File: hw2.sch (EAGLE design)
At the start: 23 parts, among them J1 USB-MB-H

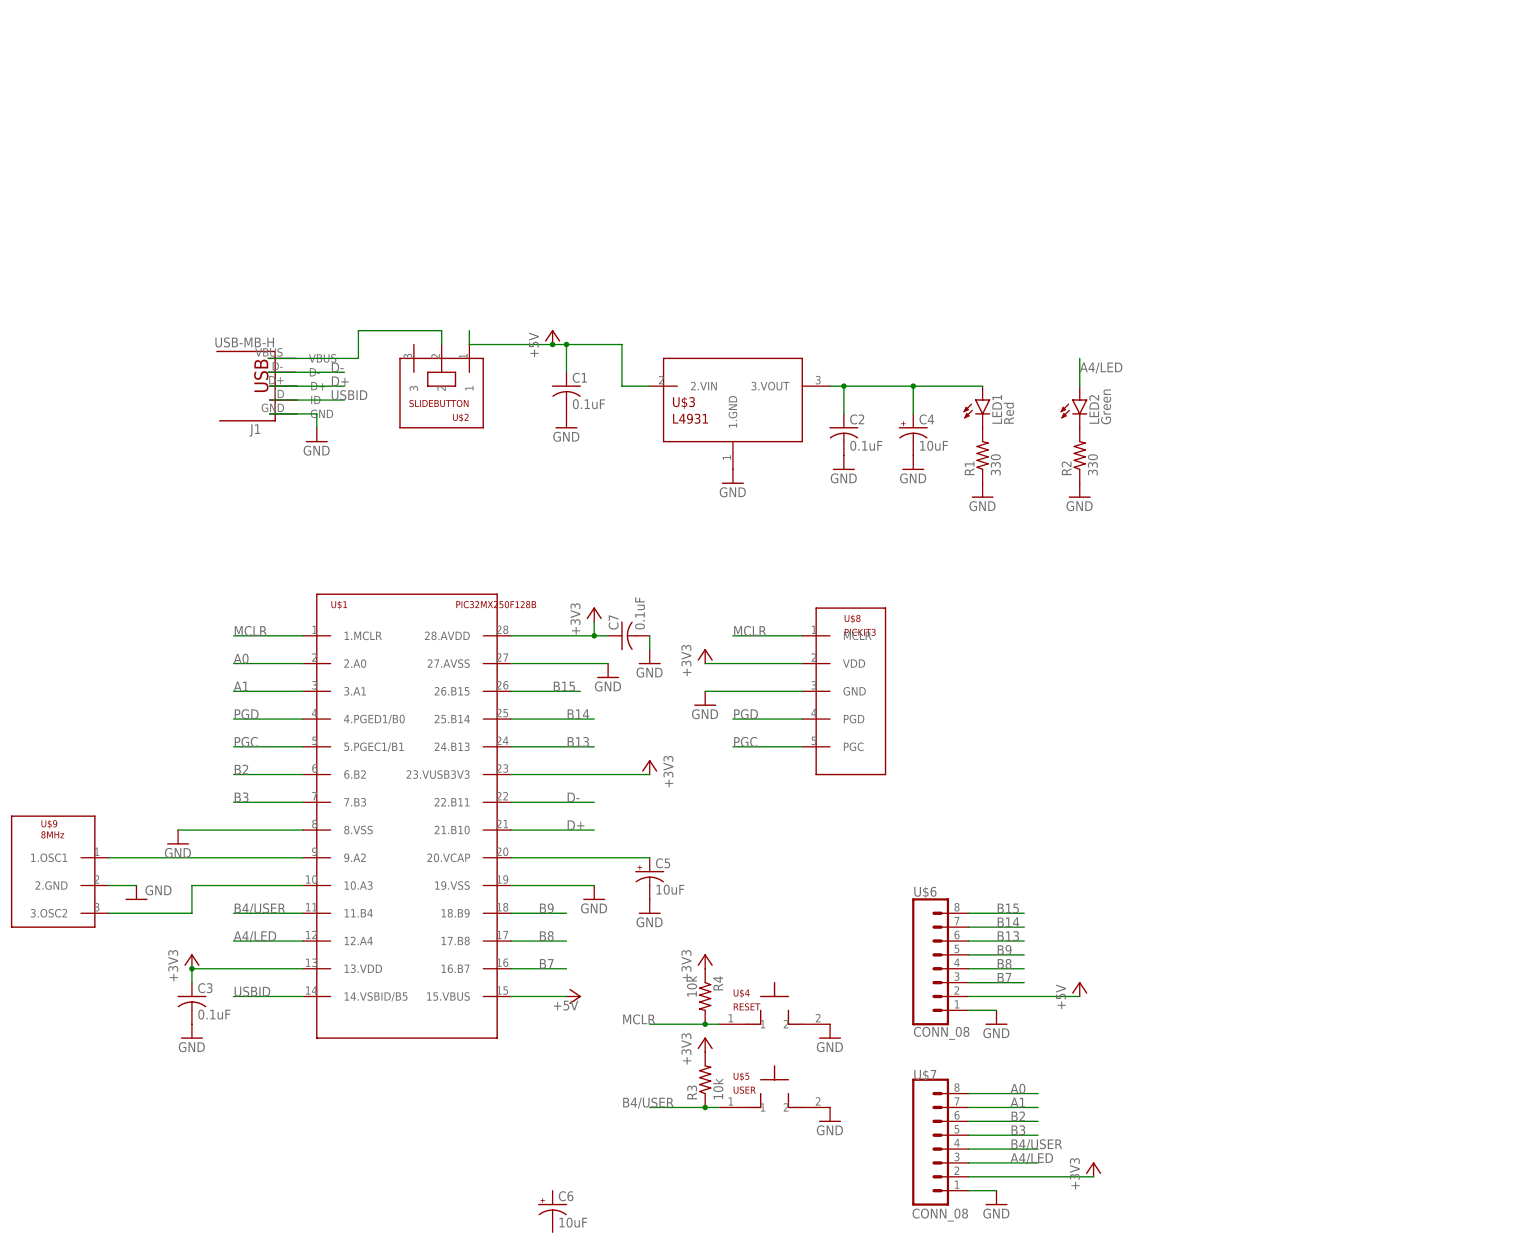
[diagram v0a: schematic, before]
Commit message: Add files via upload
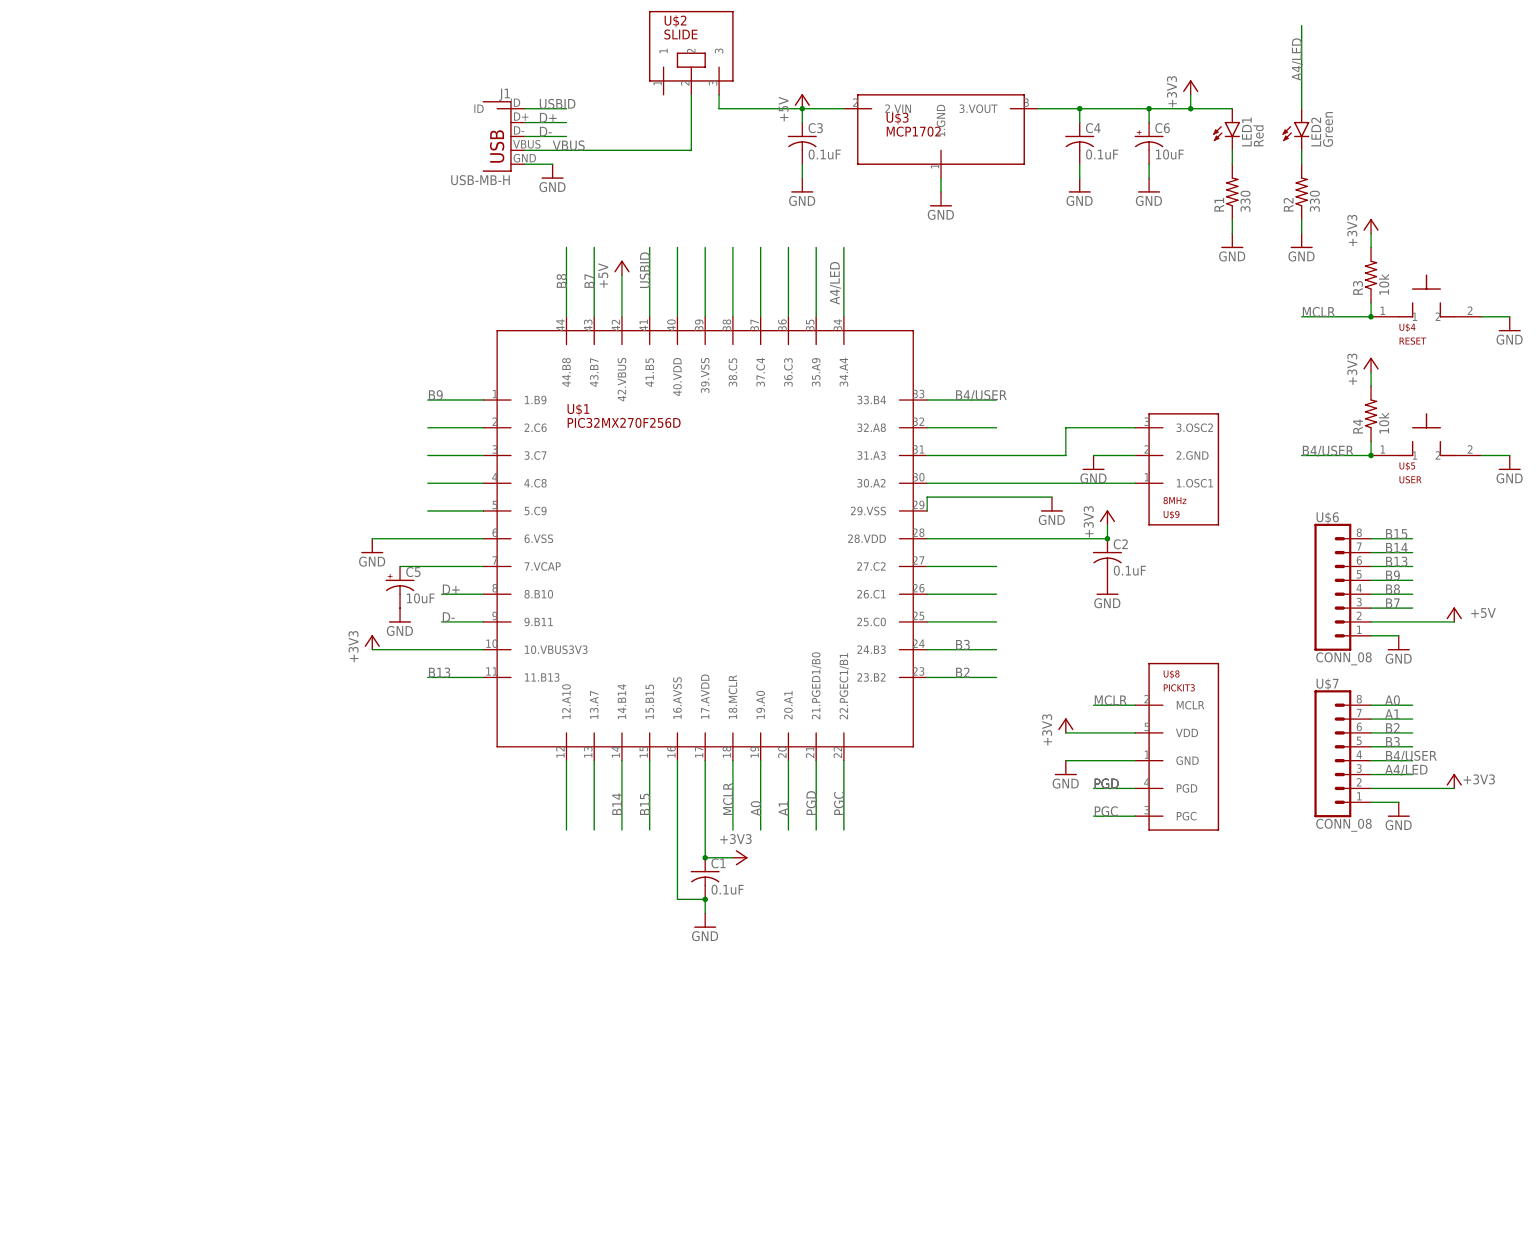
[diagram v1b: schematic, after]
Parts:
- removed C7: 0.1uF, me433:C-US025-025X050
- C1, C2, C3: device me433:C-US025-025X050 -> hw2:C-US025-025X050
- C4: value 10uF -> 0.1uF; device me433:CPOL-USB45181B -> hw2:C-US025-025X050
- C5, C6: device me433:CPOL-USB45181B -> hw2:CPOL-USB45181B
- J1: device me433:USB-MB-H -> hw2:USB-MB-H
- LED1, LED2: device me433:LED3MM -> led:LED3MM
- R1, R2, R3, R4: device me433:R-US_0207/10 -> hw2:R-US_0207/10
- U$1: value PIC32MX250F128B -> PIC32MX270F256D; device me433:PIC32MX250F128B -> hw2:PIC32MX270F256D
- U$2: value SLIDEBUTTON -> SLIDE; device me433:SLIDEBUTTON -> hw2:SLIDE
- U$3: value L4931 -> MCP1702; device me433:L4931 -> hw2:MCP1702
- U$4, U$5: device me433:PUSHBUTTON -> hw2:PB
- U$6, U$7: device me433:CONN_08 -> hw2:CONN_08
- U$8: device me433:PICKIT3 -> hw2:PICKIT3
- U$9: device me433:OSC -> hw2:OSC
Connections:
- net N$1 renamed VBUS
- removed net N$8: C5.+, U$1.20.VCAP
- new net N$10: U$1.3.C7
- new net N$11: U$1.4.C8
- new net N$12: U$1.5.C9
- new net N$17: U$1.12.A10
- new net N$18: U$1.13.A7
- new net N$27: U$1.27.C2
- new net N$28: U$1.26.C1
- new net N$29: U$1.25.C0
- new net N$35: U$1.40.VDD
- new net N$36: U$1.39.VSS
- new net N$37: U$1.38.C5
- new net N$38: U$1.37.C4
- new net N$39: U$1.36.C3
- new net N$40: U$1.35.A9
- new net N$6: U$1.32.A8
- new net N$9: U$1.2.C6
- net +3V3: now also C1.1, C2.1, C4.1, C6.+, LED1.A, R3.2, R4.2, U$1.10.VBUS3V3, U$1.17.AVDD, U$1.28.VDD, U$3.3.VOUT; no longer C3.1, C7.1, R4.1, U$1.13.VDD, U$1.23.VUSB3V3, U$1.28.AVDD
- net +5V: now also C3.1, U$1.42.VBUS, U$2.3; no longer C1.1, U$1.15.VBUS, U$2.1
- net A0: now also U$1.19.A0; no longer U$1.2.A0
- net A1: now also U$1.20.A1; no longer U$1.3.A1
- net A4/LED: now also U$1.34.A4; no longer U$1.12.A4
- net B13: now also U$1.11.B13; no longer U$1.24.B13
- net B14: now also U$1.14.B14; no longer U$1.25.B14
- net B15: now also U$1.15.B15; no longer U$1.26.B15
- net B2: now also U$1.23.B2; no longer U$1.6.B2
- net B3: now also U$1.24.B3; no longer U$1.7.B3
- net B4/USER: now also R4.1, U$1.33.B4; no longer R3.1, R3.2, U$1.11.B4
- net B7: now also U$1.43.B7; no longer U$1.16.B7
- net B8: now also U$1.44.B8; no longer U$1.17.B8
- net B9: now also U$1.1.B9; no longer U$1.18.B9
- net D+: now also U$1.8.B10; no longer U$1.21.B10
- net D-: now also U$1.9.B11; no longer U$1.22.B11
- net GND: now also C4.2, C6.-, U$1.16.AVSS, U$1.29.VSS, U$1.6.VSS; no longer C4.-, C7.2, U$1.19.VSS, U$1.27.AVSS, U$1.8.VSS
- net MCLR: now also R3.1, U$1.18.MCLR; no longer R4.2, U$1.1.MCLR
- net N$2: now also C5.+, U$1.7.VCAP; no longer C2.1, C4.+, LED1.A, U$3.3.VOUT
- net N$4: now also U$1.30.A2; no longer U$1.9.A2
- net N$5: now also U$1.31.A3; no longer U$1.10.A3
- net PGC: now also U$1.22.PGEC1/B1; no longer U$1.5.PGEC1/B1
- net PGD: now also U$1.21.PGED1/B0; no longer U$1.4.PGED1/B0
- net USBID: now also U$1.41.B5; no longer U$1.14.VSBID/B5
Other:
- moved on the sheet: C1, C2, C3, C5, C6, LED1, LED2, R1, R2, R3, R4, U$2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
